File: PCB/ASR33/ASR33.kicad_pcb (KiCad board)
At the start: 2 copper layers, 45 x 24.5 mm, 36 parts, among them J2 DC, J3 Power, J4 RUN, J5 Tx, J6 Rx, J7 USB-C, J8 Shelly, Q1 NX7002AK, SW1 SW_Push, U1 MD8942, U3 NCR402U, U4 NCR402U, U5 LTV-356T, U7 QR, U8 ESP32-S3-MINI-1

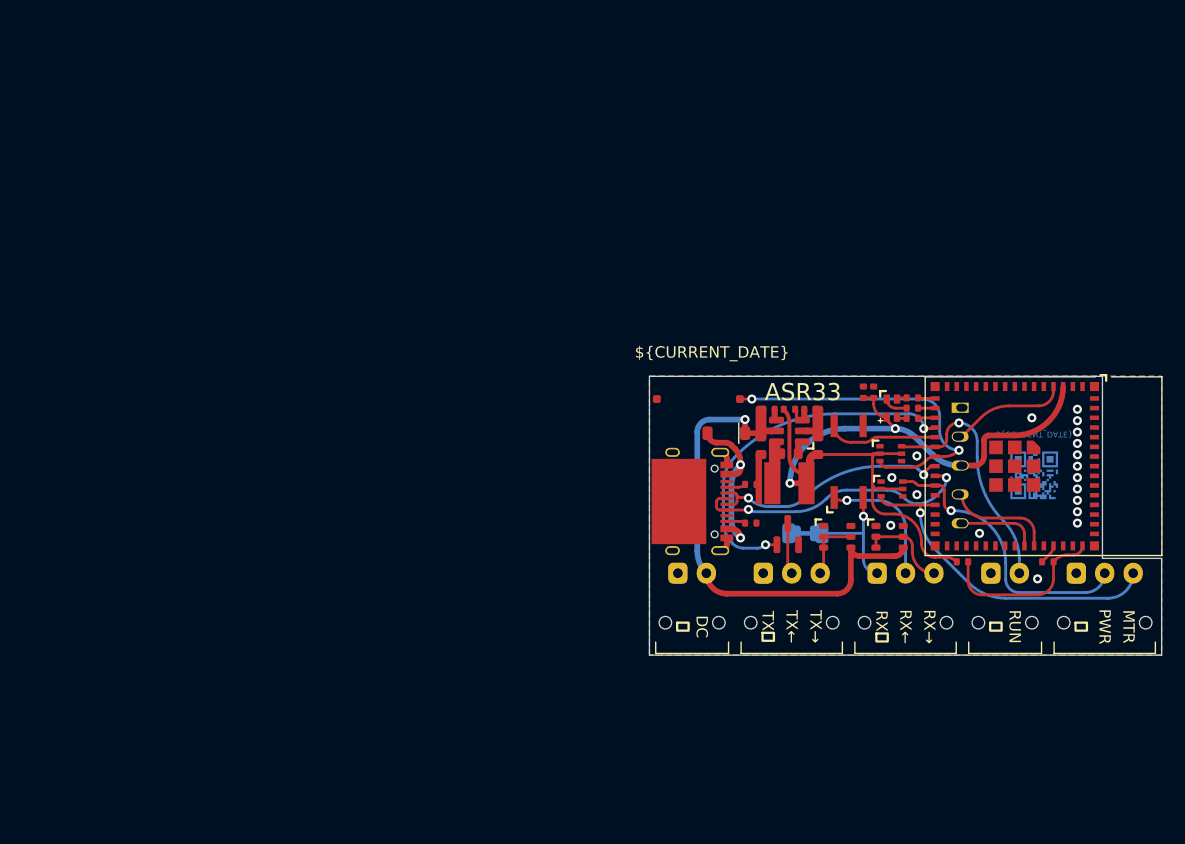
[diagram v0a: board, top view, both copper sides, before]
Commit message: Clean up PCB
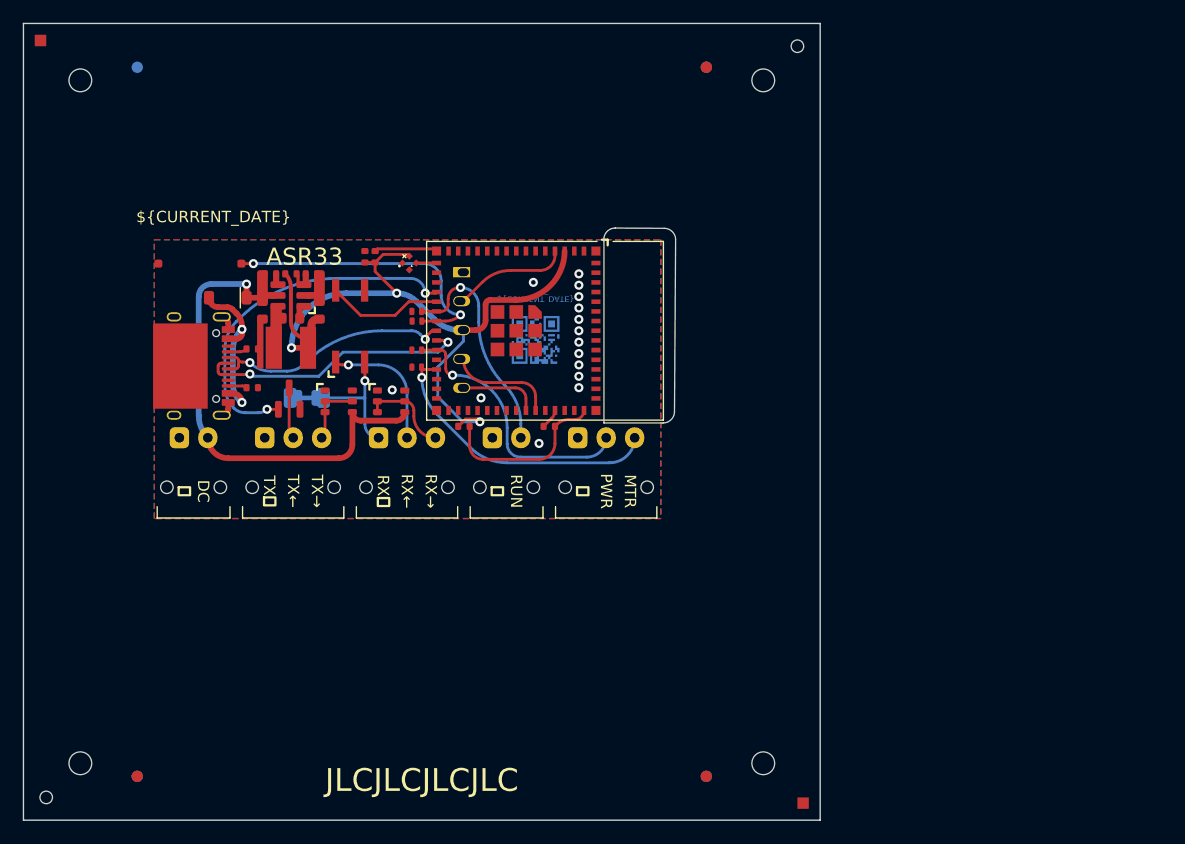
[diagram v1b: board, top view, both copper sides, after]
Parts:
- removed D5: RGB, RevK:LED-RGB-1.6x1.6
- removed R11: 680R, RevK:R_0402
- removed R12: 2K, RevK:R_0402
- removed R14: 220R, RevK:R_0402
- added D4: XL-1010RGBC-WS2812B, RevK:SMD1010, F.Cu at (98.9, 86.0)
- added D6: ~, RevK:DFN1006-2L, F.Cu at (99.5, 95.2)
- added D7: ~, RevK:DFN1006-2L, F.Cu at (99.5, 90.3)
- added PCB1: 70x70, RevK:PCB7070, F.Cu at (100.0, 100.0)
- added V1: ~, RevK:VCUT70N, F.Cu at (100.0, 84.0)
- added V2: ~, RevK:VCUT70N, F.Cu at (100.0, 108.5)
- added V3: ~, RevK:VCUT70N, F.Cu at (76.5, 100.0)
- added V4: ~, RevK:VCUT70N, F.Cu at (121.0, 100.0)
- D2, D3: value BAV99S -> ~; footprint RevK:SOT-363_SC-70-6 -> RevK:DFN1006-2L
- J7: value USB-C -> USB-C-Socket-V; footprint RevK:USC16-TR -> RevK:USB-C-Socket-H
- moved C1 45.4 mm to (86.0, 90.2)
- moved C10 45.4 mm to (95.0, 85.5)
- moved C12 45.4 mm to (88.5, 90.9)
- moved C8 45.4 mm to (91.0, 90.2)
- moved J8 45.4 mm to (103.5, 91.9)
- moved L2 45.4 mm to (88.5, 93.5)
- moved Q1 45.4 mm to (88.3, 98.0)
- moved R1 45.4 mm to (88.5, 87.0)
- moved R7 45.4 mm to (85.1, 93.6)
- moved R8 45.4 mm to (85.1, 97.0)
- moved U1 45.4 mm to (88.5, 88.9)
- moved U7 45.4 mm to (110.0, 92.8)
- moved C11 45.4 mm to (111.2, 100.4)
- moved D1 45.4 mm to (83.0, 89.1)
- moved J2 45.4 mm to (80.0, 101.4)
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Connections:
- D2 pad 1: GND -> BUTTON
- D2 pad 2: +3V3 -> GND
- D3 pad 1: GND -> PWR
- D3 pad 2: +3V3 -> GND
- U8 pad 16: G -> RGB
- U8 pad 17: R -> unconnected-(U8-GPIO13-Pad17)
- U8 pad 18: B -> unconnected-(U8-GPIO14-Pad18)
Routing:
- net +3V3: track 63.0 -> 54.8 mm, vias 2 -> 3
- net GND: track 4.62 -> 10.2 mm, vias 18 -> 15
- net BUTTON: track 29.9 -> 25.8 mm
- net MTR: track 29.5 -> 25.6 mm
- net Net-(D5-RK): track 2.17 -> 0.00 mm
- net RGB: track 0.00 -> 1.80 mm
- net PWR: track 25.0 -> 23.4 mm
- net RUN: track 21.3 -> 19.7 mm
- net R: track 1.50 -> 0.00 mm
- net G: track 1.45 -> 0.00 mm
- net B: track 1.45 -> 0.00 mm
- net Net-(D5-GK): track 0.75 -> 0.00 mm
- net Net-(D5-BK): track 0.75 -> 0.00 mm
- net D+: track 24.9 -> 24.2 mm
- net RX20MA: track 9.75 -> 10.3 mm
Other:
- board size 45 x 24.5 mm -> 70 x 70 mm
- board text added: "RGB:12"
- board text removed: "RGB: 13/2/14"
